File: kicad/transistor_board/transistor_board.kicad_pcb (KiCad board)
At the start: 2 copper layers, 25.4 x 40.6 mm, 16 parts, among them J1 Conn_01x10, J2 Conn_01x02, Q1 MMBF170, Q2 MMBF170, Q3 MMBF170, Q4 MMBF170, U2 ESP32-cam, U3 LM7805_TO220

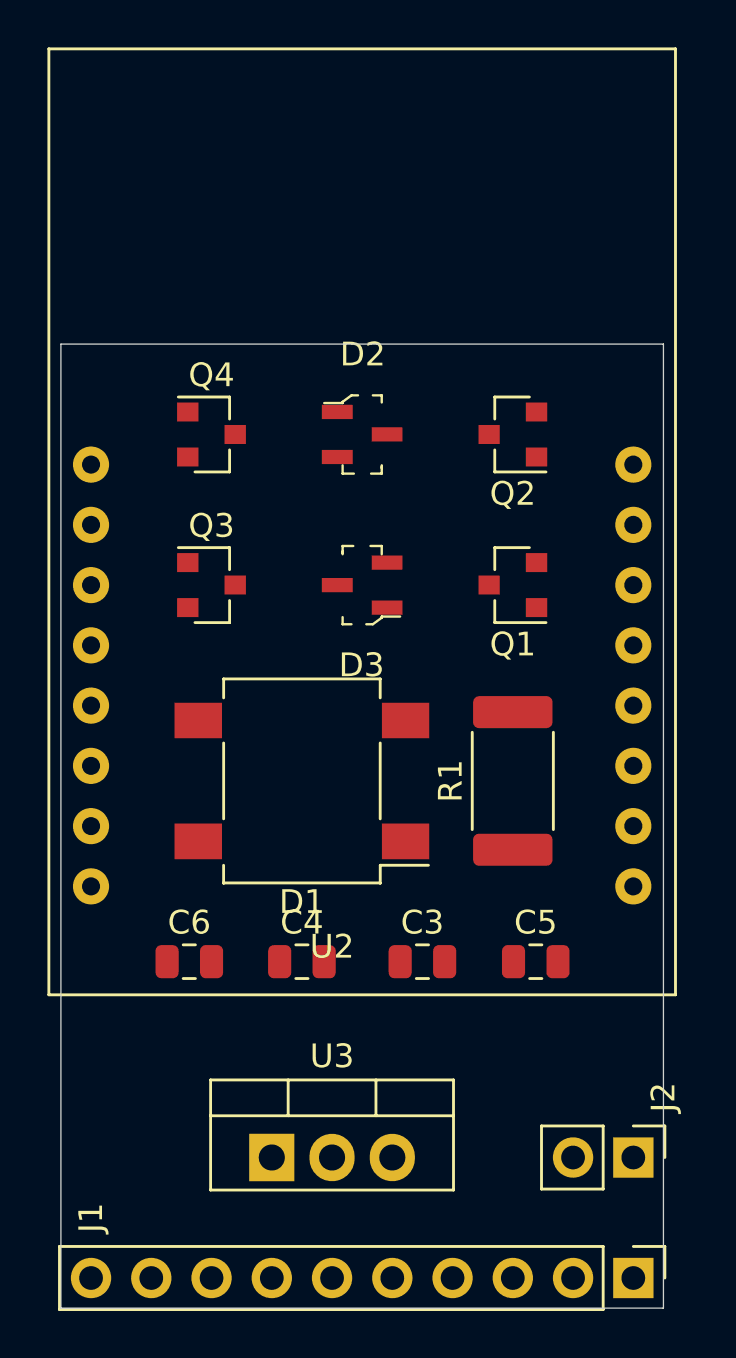
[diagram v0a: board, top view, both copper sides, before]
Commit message: routed all
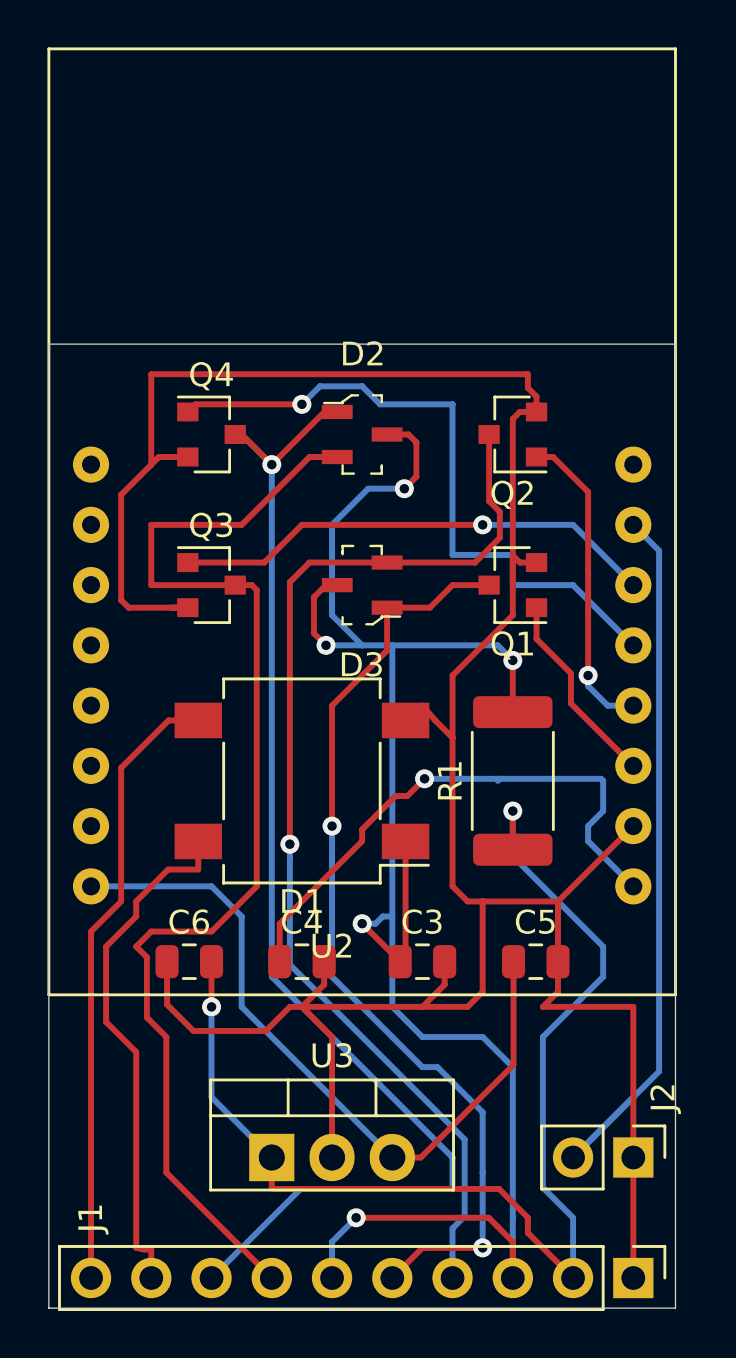
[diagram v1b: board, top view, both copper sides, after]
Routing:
- net GND: track 0.00 -> 119.5 mm
- net Net-(C3-Pad1): track 0.00 -> 79.1 mm, vias 0 -> 5
- net Net-(D2-Pad1): track 0.00 -> 52.9 mm, vias 0 -> 1
- net Net-(D2-Pad2): track 0.00 -> 51.1 mm
- net Net-(C6-Pad2): track 0.00 -> 50.0 mm, vias 0 -> 2
- net Net-(D3-Pad2): track 0.00 -> 46.8 mm, vias 0 -> 1
- net Net-(D3-Pad1): track 0.00 -> 40.0 mm, vias 0 -> 2
- net Net-(J2-Pad2): track 0.00 -> 32.2 mm
- net Net-(C5-Pad1): track 0.00 -> 31.4 mm
- net Net-(Q4-Pad1): track 0.00 -> 28.3 mm, vias 0 -> 1
- net Net-(D1-Pad3): track 0.00 -> 26.2 mm
- net Net-(C4-Pad1): track 0.00 -> 23.7 mm, vias 0 -> 1
- net Net-(D1-Pad4): track 0.00 -> 21.9 mm
- net Net-(Q3-Pad1): track 0.00 -> 20.5 mm, vias 0 -> 1
- net Net-(Q2-Pad1): track 0.00 -> 13.2 mm, vias 0 -> 1
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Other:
- board size 25.4 x 40.6 mm -> 26.4 x 40.6 mm
